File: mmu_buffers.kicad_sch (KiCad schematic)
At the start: 7 parts, among them U1 74HC541, U17 74HC04, U2 74HC541, U3 74HC245, U6 74HC541, U7 74HC541, U8 74HC245

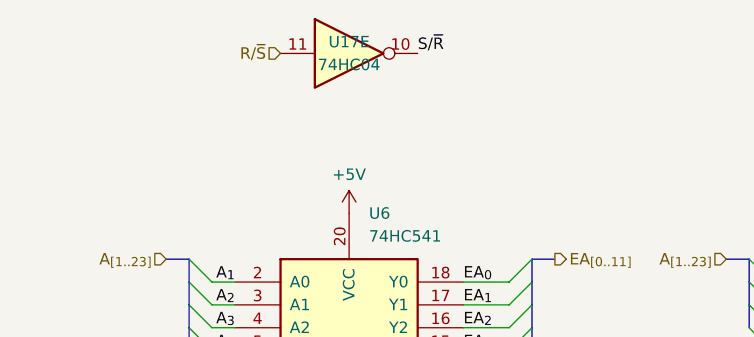
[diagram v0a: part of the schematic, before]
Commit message: applied sf68 & ps2 fixes stash from master
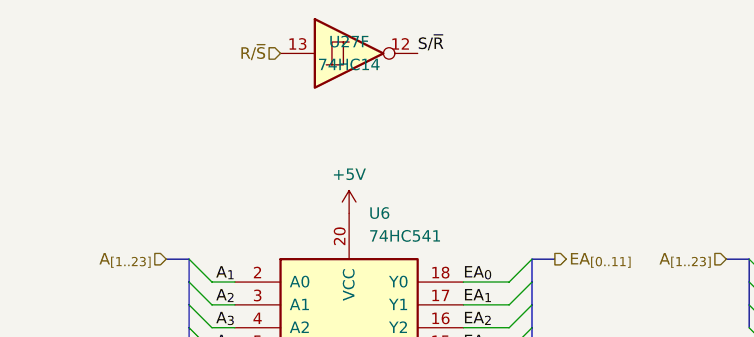
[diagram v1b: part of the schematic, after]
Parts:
- removed U17: 74HC04, Package_DIP:DIP-14_W7.62mm, symbol 74xx:74LS04
- added U27: 74HC14, Package_DIP:DIP-14_W7.62mm, symbol 74xx:74HC14
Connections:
- net R/~{S}: now also U27.13
- net S/~{R}: now also U27.12
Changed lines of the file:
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@@
-	)
-	(symbol
-		(lib_id "74xx:74LS04")
-		(at 50.8 38.1 0)
-		(unit 5)
-		(exclude_from_sim no)
-		(in_bom yes)
-		(on_board yes)
-		(dnp no)
-		(property "Reference" "U17"
-			(at 50.8 36.83 0)
-			(effects
-				(font
-					(size 1.27 1.27)
-				)
-			)
-		)
-		(property "Value" "74HC04"
-			(at 50.8 39.37 0)
-			(effects
-				(font
-					(size 1.27 1.27)
-				)
-			)
-		)
-		(property "Footprint" "Package_DIP:DIP-14_W7.62mm"
-			(at 50.8 38.1 0)
-			(effects
-				(font
-					(size 1.27 1.27)
-				)
-				(hide yes)
-			)
-		)
-		(property "Datasheet" ""
-			(at 50.8 38.1 0)
-			(effects
-				(font
-					(size 1.27 1.27)
-				)
-				(hide yes)
-			)
-		)
-		(property "Description" ""
-			(at 50.8 38.1 0)
-			(effects
-				(font
-					(size 1.27 1.27)
-				)
-				(hide yes)
-			)
-		)
-		(pin "5"
-		)
-		(pin "4"
-		)
-		(pin "13"
-		)
-		(pin "1"
-		)
-		(pin "14"
-		)
-		(pin "3"
-		)
-		(pin "6"
-		)
-		(pin "8"
-		)
-		(pin "11"
-		)
-		(pin "12"
-		)
-		(pin "7"
-		)
-		(pin "2"
-		)
-		(pin "9"
-		)
-		(pin "10"
-		)
-		(instances
-			(project "SCRM6816"
-				(path "/56448118-82b3-4e1c-bda3-84d63e01a14a/c5c5c8e4-8884-4f58-9370-e357b3396fe5/98a6ea48-1e81-41f7-a844-db039b7dc800"
-					(reference "U17")
-					(unit 5)
-				)
-			)
-		)
 	)
 	(symbol
@@
 				)
 			)
+		)
+	)
+	(symbol
+		(lib_id "74xx:74HC14")
+		(at 50.8 38.1 0)
+		(unit 6)
+		(exclude_from_sim no)
+		(in_bom yes)
+		(on_board yes)
+		(dnp no)
+		(property "Reference" "U27"
+			(at 50.8 36.83 0)
+			(effects
+				(font
+					(size 1.27 1.27)
+				)
+			)
+		)
+		(property "Value" "74HC14"
+			(at 50.8 39.37 0)
+			(effects
+				(font
+					(size 1.27 1.27)
+				)
+			)
+		)
+		(property "Footprint" "Package_DIP:DIP-14_W7.62mm"
+			(at 50.8 38.1 0)
+			(effects
+				(font
+					(size 1.27 1.27)
+				)
+				(hide yes)
+			)
+		)
+		(property "Datasheet" ""
+			(at 50.8 38.1 0)
+			(effects
+				(font
+					(size 1.27 1.27)
+				)
+				(hide yes)
+			)
+		)
+		(property "Description" ""
+			(at 50.8 38.1 0)
+			(effects
+				(font
+					(size 1.27 1.27)
+				)
+				(hide yes)
+			)
+		)
+		(pin "1"
+		)
+		(pin "5"
+		)
+		(pin "6"
+		)
+		(pin "4"
+		)
+		(pin "2"
+		)
+		(pin "8"
+		)
+		(pin "9"
+		)
+		(pin "3"
+		)
+		(pin "12"
+		)
+		(pin "10"
+		)
+		(pin "7"
+		)
+		(pin "13"
+		)
+		(pin "14"
+		)
+		(pin "11"
+		)
+		(instances
+			(project "SF68"
+				(path "/56448118-82b3-4e1c-bda3-84d63e01a14a/c5c5c8e4-8884-4f58-9370-e357b3396fe5/98a6ea48-1e81-41f7-a844-db039b7dc800"
+					(reference "U27")
+					(unit 6)
+				)
+			)
